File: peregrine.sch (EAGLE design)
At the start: 77 parts, among them J1 USB MICRO, Q1 BSS123, Q10 BSS123, Q11 BSS123, Q2 BSS123, U1 ITG-3200, U2 ADXL345, U5 ATMEGA32U4-XUAU, Y1 16MHz KX-7

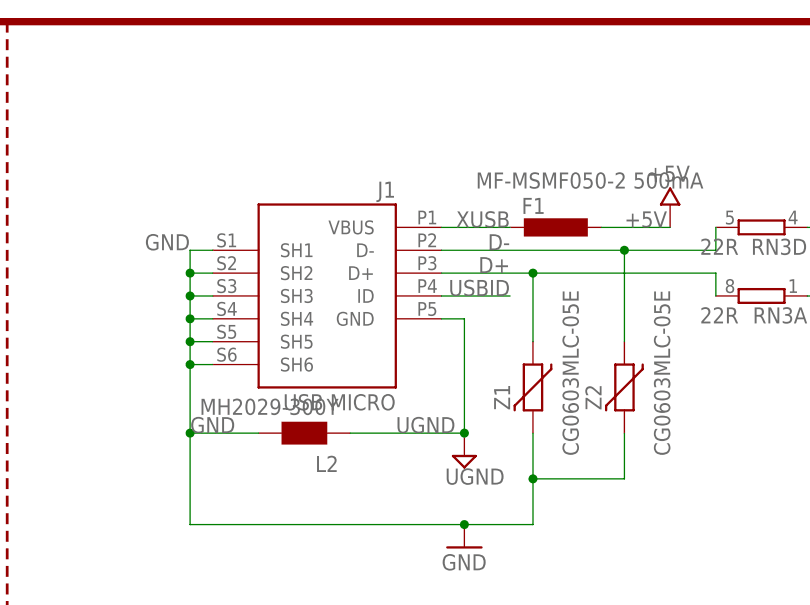
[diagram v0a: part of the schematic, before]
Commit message: Not a change, Just including version of board which was sent out.
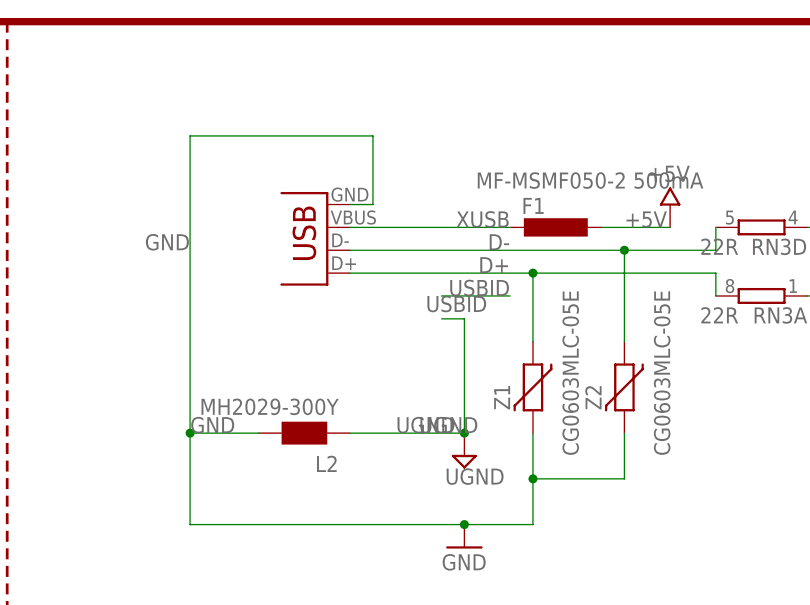
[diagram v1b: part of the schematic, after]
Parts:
- removed J1: USB MICRO, SmartPrj:MYCON2_USB-MINI-B
- added X2: USB-MICROB, SparkFun:USB-MICROB
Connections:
- removed net USBID: J1.ID
- net D+: now also X2.D+; no longer J1.D+
- net D-: now also X2.D-; no longer J1.D-
- net GND: now also X2.GND; no longer J1.SH1, J1.SH2, J1.SH3, J1.SH4, J1.SH5, J1.SH6
- net UGND: no longer J1.GND
- net XUSB: now also X2.VBUS; no longer J1.VBUS
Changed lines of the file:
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@@
 <part name="Y1" library="SmartPrj" deviceset="CRYSTAL-3.2-2.5" device="" value="16MHz KX-7"/>
 <part name="D2" library="diode" deviceset="DIODE-" device="MINIMELF" value="CD1206-S01575"/>
-<part name="J1" library="SmartPrj" deviceset="MYCON2_USB-MINI-B" device="" value="USB MICRO"/>
 <part name="GND51" library="supply1" deviceset="GND" device=""/>
 <part name="U$3" library="SparkFun" deviceset="BMP085" device=""/>
@@
 <part name="GND17" library="SparkFun" deviceset="GND" device=""/>
 <part name="GND19" library="SparkFun" deviceset="GND" device=""/>
+<part name="X2" library="SparkFun" deviceset="USB" device="-MICROB"/>
 </parts>
 <sheets>
@@
 <attribute name="VALUE" x="-119.6086" y="152.4" size="1.778" layer="96" rot="R90"/>
 </instance>
-<instance part="J1" gate="G$1" x="175.26" y="175.26" rot="MR0"/>
 <instance part="GND51" gate="1" x="190.5" y="144.78"/>
 <instance part="U$3" gate="G$1" x="-40.64" y="-33.02"/>
@@
 <instance part="GND17" gate="1" x="88.9" y="71.12"/>
 <instance part="GND19" gate="1" x="88.9" y="78.74"/>
+<instance part="X2" gate="G$1" x="175.26" y="182.88" rot="R180"/>
 </instances>
 <busses>
@@
 </segment>
 <segment>
-<wire x1="162.56" y1="170.18" x2="160.02" y2="170.18" width="0.1524" layer="91"/>
-<wire x1="160.02" y1="172.72" x2="160.02" y2="170.18" width="0.1524" layer="91"/>
-<wire x1="162.56" y1="172.72" x2="160.02" y2="172.72" width="0.1524" layer="91"/>
-<wire x1="160.02" y1="175.26" x2="160.02" y2="172.72" width="0.1524" layer="91"/>
-<wire x1="162.56" y1="175.26" x2="160.02" y2="175.26" width="0.1524" layer="91"/>
-<wire x1="160.02" y1="177.8" x2="160.02" y2="175.26" width="0.1524" layer="91"/>
-<wire x1="162.56" y1="177.8" x2="160.02" y2="177.8" width="0.1524" layer="91"/>
 <wire x1="198.12" y1="152.4" x2="198.12" y2="147.32" width="0.1524" layer="91"/>
 <wire x1="198.12" y1="152.4" x2="198.12" y2="157.48" width="0.1524" layer="91"/>
@@
 <wire x1="208.28" y1="157.48" x2="208.28" y2="152.4" width="0.1524" layer="91"/>
 <wire x1="167.64" y1="157.48" x2="160.02" y2="157.48" width="0.1524" layer="91"/>
-<wire x1="160.02" y1="157.48" x2="160.02" y2="165.1" width="0.1524" layer="91"/>
-<wire x1="160.02" y1="165.1" x2="160.02" y2="167.64" width="0.1524" layer="91"/>
-<wire x1="160.02" y1="167.64" x2="160.02" y2="170.18" width="0.1524" layer="91"/>
 <wire x1="198.12" y1="147.32" x2="190.5" y2="147.32" width="0.1524" layer="91"/>
 <wire x1="190.5" y1="147.32" x2="160.02" y2="147.32" width="0.1524" layer="91"/>
 <wire x1="160.02" y1="147.32" x2="160.02" y2="157.48" width="0.1524" layer="91"/>
-<wire x1="162.56" y1="167.64" x2="160.02" y2="167.64" width="0.1524" layer="91"/>
-<wire x1="162.56" y1="165.1" x2="160.02" y2="165.1" width="0.1524" layer="91"/>
-<junction x="160.02" y="172.72"/>
-<junction x="160.02" y="175.26"/>
 <junction x="198.12" y="152.4"/>
-<junction x="160.02" y="170.18"/>
 <junction x="160.02" y="157.48"/>
-<junction x="160.02" y="167.64"/>
-<junction x="160.02" y="165.1"/>
 <junction x="190.5" y="147.32"/>
 <label x="160.02" y="177.8" size="1.778" layer="95" rot="MR0"/>
@@
 <pinref part="L2" gate="G$1" pin="2"/>
 <pinref part="Z2" gate="G$1" pin="2"/>
-<pinref part="J1" gate="G$1" pin="SH1"/>
-<pinref part="J1" gate="G$1" pin="SH2"/>
-<pinref part="J1" gate="G$1" pin="SH3"/>
-<pinref part="J1" gate="G$1" pin="SH4"/>
-<pinref part="J1" gate="G$1" pin="SH5"/>
-<pinref part="J1" gate="G$1" pin="SH6"/>
 <pinref part="GND51" gate="1" pin="GND"/>
+<pinref part="X2" gate="G$1" pin="GND"/>
+<wire x1="177.8" y1="182.88" x2="180.34" y2="182.88" width="0.1524" layer="91"/>
+<wire x1="180.34" y1="182.88" x2="180.34" y2="190.5" width="0.1524" layer="91"/>
+<wire x1="180.34" y1="190.5" x2="160.02" y2="190.5" width="0.1524" layer="91"/>
+<wire x1="160.02" y1="190.5" x2="160.02" y2="157.48" width="0.1524" layer="91"/>
 </segment>
 <segment>
@@
 <segment>
 <wire x1="218.44" y1="177.8" x2="208.28" y2="177.8" width="0.1524" layer="91"/>
-<wire x1="208.28" y1="177.8" x2="187.96" y2="177.8" width="0.1524" layer="91"/>
+<wire x1="208.28" y1="177.8" x2="177.8" y2="177.8" width="0.1524" layer="91"/>
 <wire x1="218.44" y1="177.8" x2="218.44" y2="180.34" width="0.1524" layer="91"/>
 <wire x1="208.28" y1="167.64" x2="208.28" y2="177.8" width="0.1524" layer="91"/>
@@
 <pinref part="Z2" gate="G$1" pin="1"/>
 <pinref part="RN3" gate="D" pin="2"/>
-<pinref part="J1" gate="G$1" pin="D-"/>
+<pinref part="X2" gate="G$1" pin="D-"/>
 </segment>
 </net>
@@
 <segment>
 <wire x1="218.44" y1="175.26" x2="198.12" y2="175.26" width="0.1524" layer="91"/>
-<wire x1="198.12" y1="175.26" x2="187.96" y2="175.26" width="0.1524" layer="91"/>
 <wire x1="218.44" y1="175.26" x2="218.44" y2="172.72" width="0.1524" layer="91"/>
 <wire x1="198.12" y1="167.64" x2="198.12" y2="175.26" width="0.1524" layer="91"/>
@@
 <pinref part="Z1" gate="G$1" pin="1"/>
 <pinref part="RN3" gate="A" pin="2"/>
-<pinref part="J1" gate="G$1" pin="D+"/>
+<pinref part="X2" gate="G$1" pin="D+"/>
+<wire x1="198.12" y1="175.26" x2="177.8" y2="175.26" width="0.1524" layer="91"/>
 </segment>
 </net>
@@
 <pinref part="L2" gate="G$1" pin="1"/>
 <pinref part="SUPPLY1" gate="G$1" pin="GND1"/>
-<pinref part="J1" gate="G$1" pin="GND"/>
+<label x="185.42" y="157.48" size="1.778" layer="95"/>
 </segment>
 </net>
 <net name="XUSB" class="3">
 <segment>
-<wire x1="187.96" y1="180.34" x2="195.58" y2="180.34" width="0.1524" layer="91"/>
 <label x="195.58" y="180.34" size="1.778" layer="95" rot="MR0"/>
 <pinref part="F1" gate="G$1" pin="2"/>
-<pinref part="J1" gate="G$1" pin="VBUS"/>
+<pinref part="X2" gate="G$1" pin="VBUS"/>
+<wire x1="195.58" y1="180.34" x2="177.8" y2="180.34" width="0.1524" layer="91"/>
 </segment>
 </net>
@@
 <wire x1="195.58" y1="172.72" x2="187.96" y2="172.72" width="0.1524" layer="91"/>
 <label x="195.58" y="172.72" size="1.778" layer="95" rot="MR0"/>
-<pinref part="J1" gate="G$1" pin="ID"/>
-</segment>
-</net>
+<label x="193.04" y="172.72" size="1.778" layer="95" rot="R180"/>
+</segment>
+</net>
